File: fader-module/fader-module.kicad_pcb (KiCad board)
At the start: 2 copper layers, 100 x 75 mm, 34 parts, among them J1 Conn_1x05_Pin, J2 Conn_1x05_Socket, J3 Conn_01x02_Pin, J4 Conn_01x06_Pin, J6 Conn_01x06_Pin, SW1 1825910-6, SW2 1825910-6, U5 ATMEGA328P-AUR, U7 DRV8871DDAR

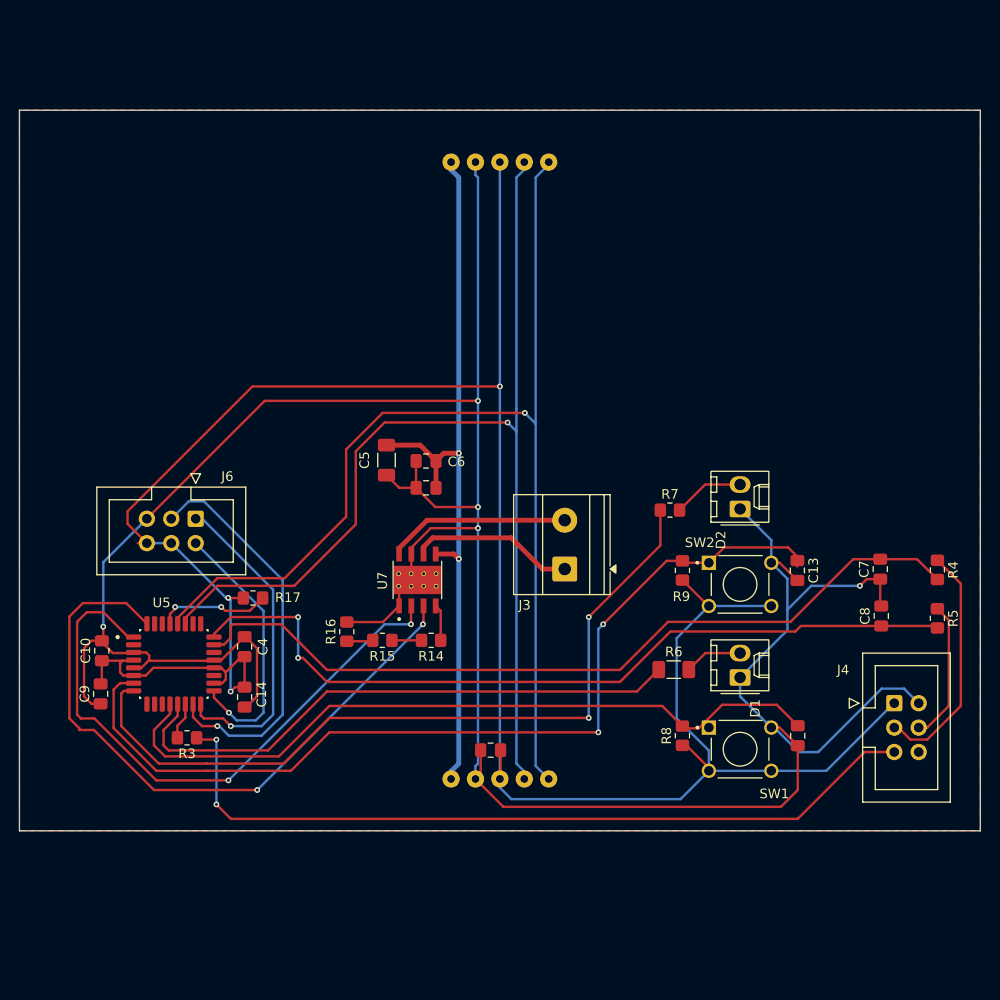
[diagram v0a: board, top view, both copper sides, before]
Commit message: done w pcb gerbert time
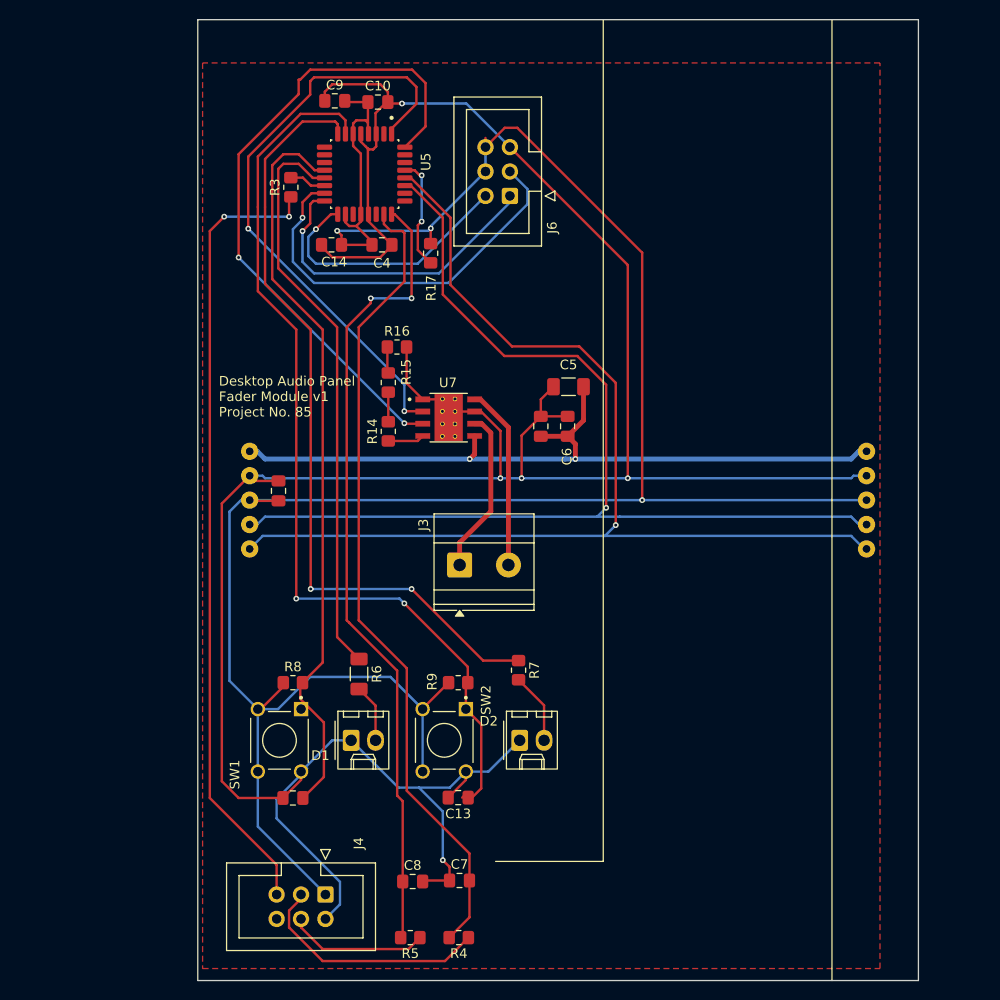
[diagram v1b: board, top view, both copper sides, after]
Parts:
- moved C9 66.4 mm to (142.8, 47.5), turned to 180 degrees
- moved R5 64.1 mm to (150.7, 134.6), turned to 180 degrees
- moved C10 63.9 mm to (147.3, 47.7), turned to 0 degrees
- moved R4 62.8 mm to (155.7, 134.6), turned to 180 degrees
- moved J4 62.5 mm to (141.8, 130.1), turned to -90 degrees
- moved R3 58.3 mm to (138.2, 56.5), turned to 90 degrees
- moved C8 56.1 mm to (150.9, 128.8), turned to 0 degrees
- moved U5 54.7 mm to (145.9, 55.1), turned to -90 degrees
- moved C7 54.5 mm to (155.8, 128.7), turned to 0 degrees
- moved C12 52.9 mm to (138.5, 120.1), turned to 180 degrees
- moved J2 51.9 mm to (198.2, 89.1), turned to -90 degrees
- moved SW1 47.9 mm to (137.1, 114.1), turned to -90 degrees
- moved C14 47.9 mm to (142.5, 62.5), turned to 180 degrees
- moved J6 46.9 mm to (161.0, 57.4), turned to 180 degrees
- moved C4 44.2 mm to (147.7, 62.5), turned to 0 degrees
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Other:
- board size 100 x 75 mm -> 75 x 100 mm
- rule pad_to_mask_clearance: 0 -> 0.05
- board text added: "Desktop Audio Panel Fader Module v1 Project No. 85"
